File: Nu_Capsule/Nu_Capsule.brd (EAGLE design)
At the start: 10 x 15 mm, 20 parts, among them T1 2SC3324, T2 2SC3324

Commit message: updates and minor corrections
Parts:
- C5: value 4.7uF -> 1uF
- R6: value 10K -> 47K
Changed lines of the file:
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@@
 <attribute name="VALUE" x="5.232" y="3.265" size="0.65" layer="27" ratio="13" rot="R90"/>
 </element>
-<element name="C5" library="resistor" package="C0805" value="4.7uF" x="5" y="4.3" smashed="yes" rot="R270">
+<element name="C5" library="resistor" package="C0805" value="1uF" x="5" y="4.3" smashed="yes" rot="R270">
 <attribute name="VALUE" x="2.714" y="5.189" size="0.65" layer="27" ratio="13" rot="R270"/>
 </element>
-<element name="R6" library="resistor" package="R0402" value="10K" x="7" y="3.8" smashed="yes" rot="R270">
+<element name="R6" library="resistor" package="R0402" value="47K" x="7" y="3.8" smashed="yes" rot="R270">
 <attribute name="VALUE" x="4.968" y="4.435" size="0.65" layer="27" ratio="13" rot="R270"/>
 </element>

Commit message: more updates; tweaks
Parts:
- C5: value 1uF -> 4.7uF
- R6: value 47K -> 10K
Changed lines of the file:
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@@
 <attribute name="VALUE" x="5.232" y="3.265" size="0.65" layer="27" ratio="13" rot="R90"/>
 </element>
-<element name="C5" library="resistor" package="C0805" value="1uF" x="5" y="4.3" smashed="yes" rot="R270">
+<element name="C5" library="resistor" package="C0805" value="4.7uF" x="5" y="4.3" smashed="yes" rot="R270">
 <attribute name="VALUE" x="2.714" y="5.189" size="0.65" layer="27" ratio="13" rot="R270"/>
 </element>
-<element name="R6" library="resistor" package="R0402" value="47K" x="7" y="3.8" smashed="yes" rot="R270">
+<element name="R6" library="resistor" package="R0402" value="10K" x="7" y="3.8" smashed="yes" rot="R270">
 <attribute name="VALUE" x="4.968" y="4.435" size="0.65" layer="27" ratio="13" rot="R270"/>
 </element>

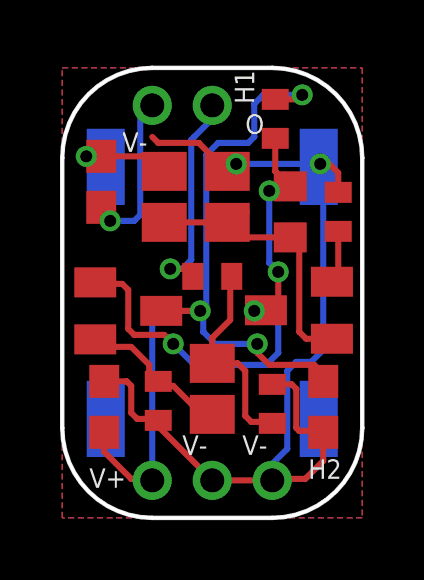
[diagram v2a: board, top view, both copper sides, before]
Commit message: Licenses
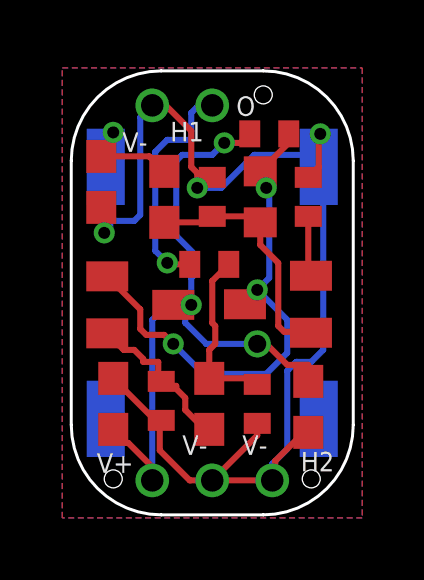
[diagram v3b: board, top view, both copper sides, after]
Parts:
- C1, C5: device resistor:C0805 -> resistor:C0603
- R2: device resistor:R0805 -> resistor:R0402
- moved R1 1.12 mm to (6.60, 10.7)
- moved R3 1.12 mm to (8.20, 10.7)
- moved T1 0.73 mm to (7.19, 7.12)
- moved R4 0.54 mm to (6.90, 12.8), turned to 180 degrees
- moved C5 0.51 mm to (4.90, 3.80)
- moved C3 0.50 mm to (8.20, 3.70)
- moved R2 0.50 mm to (5.00, 10.7)
- moved R6 0.50 mm to (6.50, 3.80), turned to 90 degrees
- moved T2 0.45 mm to (2.60, 7.10)
- moved R7 0.41 mm to (4.90, 8.45)
- moved C4 0.32 mm to (1.70, 3.80)
- moved R5 0.10 mm to (3.30, 3.90)
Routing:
- net GND: track 39.1 -> 44.2 mm
- net VIN: track 27.7 -> 24.8 mm
- net N$2: track 3.67 -> 4.88 mm
- net N$1: track 9.60 -> 8.47 mm
- net OUT: track 6.91 -> 5.83 mm
- net VCVF: track 17.9 -> 17.1 mm, vias 4 -> 3
- net OUTPUT: track 7.10 -> 7.71 mm
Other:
- board size 10 x 15 mm -> 9.4 x 14.8 mm
